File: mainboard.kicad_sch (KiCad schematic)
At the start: 0 parts

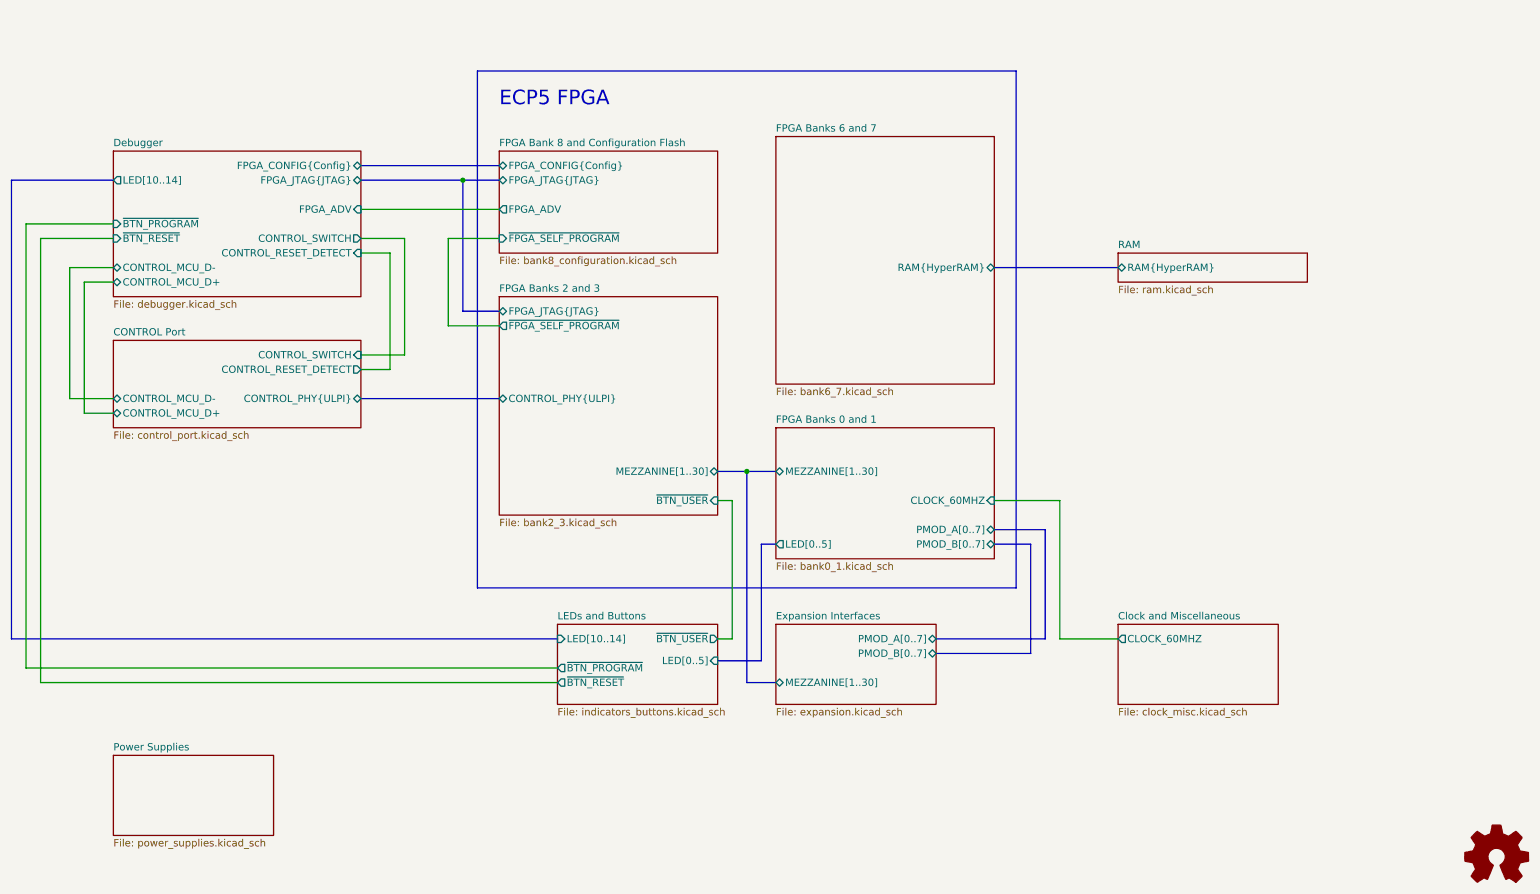
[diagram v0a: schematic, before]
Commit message: schematic wip
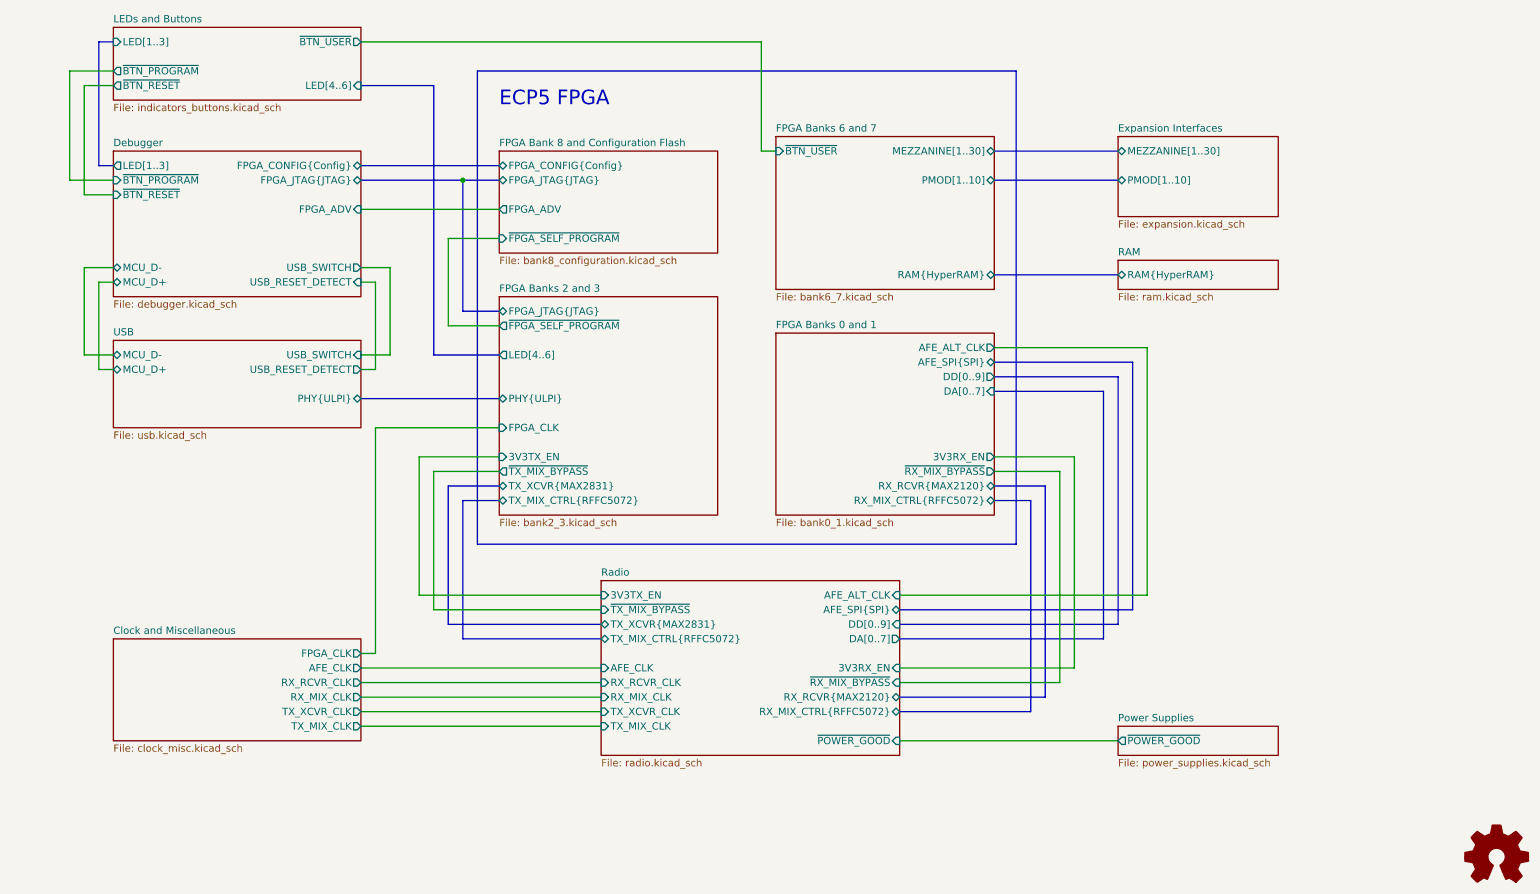
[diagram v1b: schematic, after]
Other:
- sheet CONTROL Port renamed USB
- added sheet Radio (radio.kicad_sch)
- sheet Clock and Miscellaneous ports: added AFE_CLK, FPGA_CLK, RX_MIX_CLK, RX_RCVR_CLK, TX_MIX_CLK, TX_XCVR_CLK; removed CLOCK_60MHZ
- sheet Debugger ports: added LED[1..3], MCU_D+, MCU_D-, USB_RESET_DETECT, USB_SWITCH; removed CONTROL_MCU_D+, CONTROL_MCU_D-, CONTROL_RESET_DETECT, CONTROL_SWITCH, LED[10..14]
- sheet Expansion Interfaces ports: added PMOD[1..10]; removed PMOD_A[0..7], PMOD_B[0..7]
- sheet FPGA Banks 0 and 1 ports: added 3V3RX_EN, AFE_ALT_CLK, AFE_SPI{SPI}, DA[0..7], DD[0..9], RX_MIX_CTRL{RFFC5072}, RX_RCVR{MAX2120}, ~{RX_MIX_BYPASS}; removed CLOCK_60MHZ, LED[0..5], MEZZANINE[1..30], PMOD_A[0..7], PMOD_B[0..7]
- sheet FPGA Banks 2 and 3 ports: added 3V3TX_EN, FPGA_CLK, LED[4..6], PHY{ULPI}, TX_MIX_CTRL{RFFC5072}, TX_XCVR{MAX2831}, ~{TX_MIX_BYPASS}; removed CONTROL_PHY{ULPI}, MEZZANINE[1..30], ~{BTN_USER}
- sheet FPGA Banks 6 and 7 ports: added MEZZANINE[1..30], PMOD[1..10], ~{BTN_USER}; removed none
- sheet LEDs and Buttons ports: added LED[1..3], LED[4..6]; removed LED[0..5], LED[10..14]
- sheet Power Supplies ports: added ~{POWER_GOOD}; removed none
- sheet USB: file control_port.kicad_sch -> usb.kicad_sch
- sheet USB ports: added MCU_D+, MCU_D-, PHY{ULPI}, USB_RESET_DETECT, USB_SWITCH; removed CONTROL_MCU_D+, CONTROL_MCU_D-, CONTROL_PHY{ULPI}, CONTROL_RESET_DETECT, CONTROL_SWITCH
